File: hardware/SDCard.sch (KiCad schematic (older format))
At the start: 25 parts, among them J401 Micro_SD_Card_Det, Q401 ZXTN25050DFHTA, SW1 SD SPI/MMC mode, U401 MAX4948

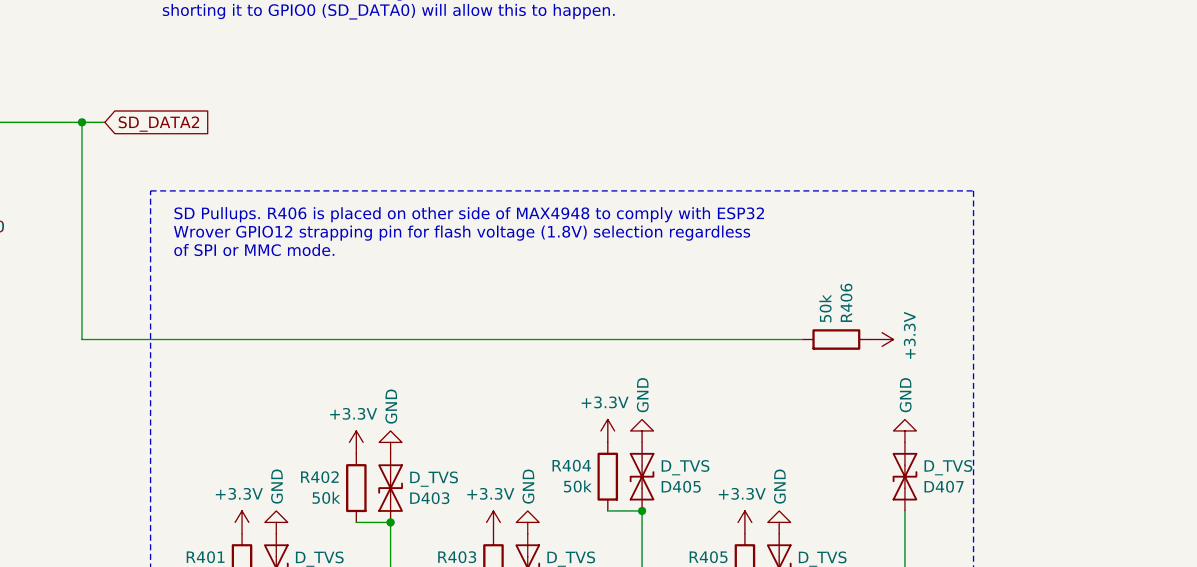
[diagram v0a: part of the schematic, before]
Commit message: Added note re. not populating R406 when using Wrover-B modules.
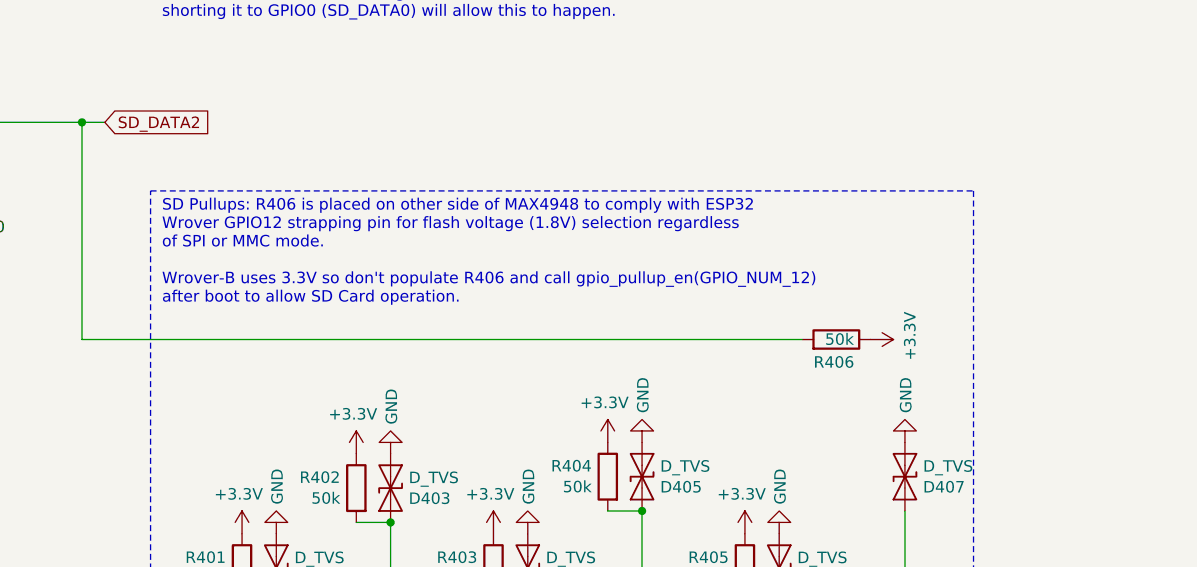
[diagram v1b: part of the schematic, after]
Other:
- note added: "SD Pullups: R406 is placed on other side of MAX4948 to comply with ESP32\nWrover GPIO12 strapping pin for flash voltage (1.8V) selection regardless\nof SPI or MMC mode.\n\nWrover-B uses 3.3V so don't populate R406 and call gpio_pullup_en(GPIO_NUM_12)\nafter boot to allow SD Card operation."
- note removed: "SD Pullups. R406 is placed on other side of MAX4948 to comply with ESP32\nWrover GPIO12 strapping pin for flash voltage (1.8V) selection regardless\nof SPI or MMC mode."
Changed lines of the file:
@@
 AR Path="/5B61FB63/5BEBC44C" Ref="R?"  Part="1"
 AR Path="/5B61FB63/5B98DF5D/5BEBC44C" Ref="R406"  Part="1"
-F 0 "R406" H 6820 2946 50  0000 L CNN
-F 1 "50k" H 6820 2855 50  0000 L CNN
+F 0 "R406" V 6650 2800 50  0000 L CNN
+F 1 "50k" V 6750 2850 50  0000 L CNN
 F 2 "Resistor_SMD:R_0805_2012Metric" V 6680 2900 50  0001 C CNN
 F 3 "https://www.mouser.se/ProductDetail/667-ERJ-6ENF5102V" H 6750 2900 50  0001 C CNN
@@
 Wire Notes Line
 	3750 2250 7350 2250
-Text Notes 3850 2550 0    50   ~ 0
-SD Pullups. R406 is placed on other side of MAX4948 to comply with ESP32\nWrover GPIO12 strapping pin for flash voltage (1.8V) selection regardless\nof SPI or MMC mode.
+Text Notes 3800 2750 0    50   ~ 0
+SD Pullups: R406 is placed on other side of MAX4948 to comply with ESP32\nWrover GPIO12 strapping pin for flash voltage (1.8V) selection regardless\nof SPI or MMC mode.\n\nWrover-B uses 3.3V so don't populate R406 and call gpio_pullup_en(GPIO_NUM_12)\nafter boot to allow SD Card operation.
 Wire Wire Line
 	3450 1950 3450 2900
